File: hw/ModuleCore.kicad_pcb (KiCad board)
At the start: 2 copper layers, 38.1 x 99.1 mm, 24 parts, among them J6 power_bus, J8 Conn_02x09_Odd_Even, Q1 2SC1815, SW5 SW_Push, U1 TL074, U2 ProMicro, U3 74HC595

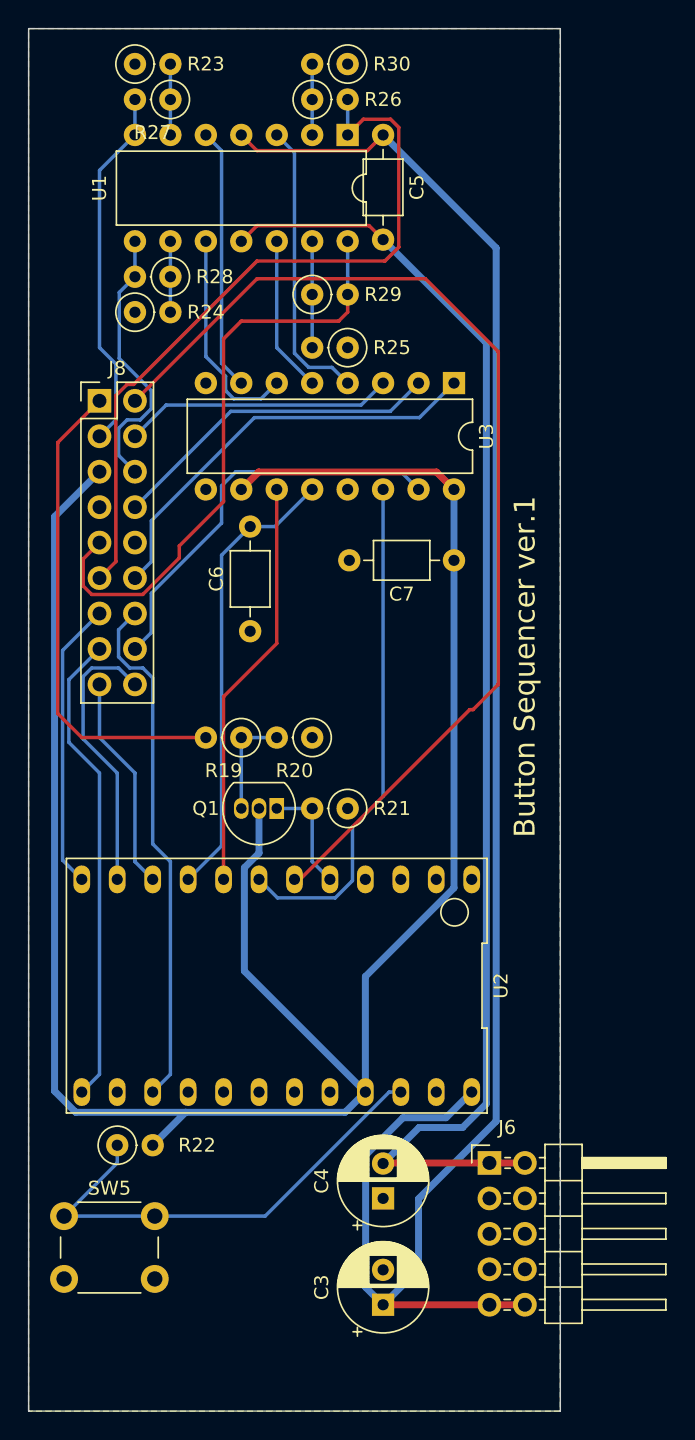
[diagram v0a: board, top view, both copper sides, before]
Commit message: minor mods
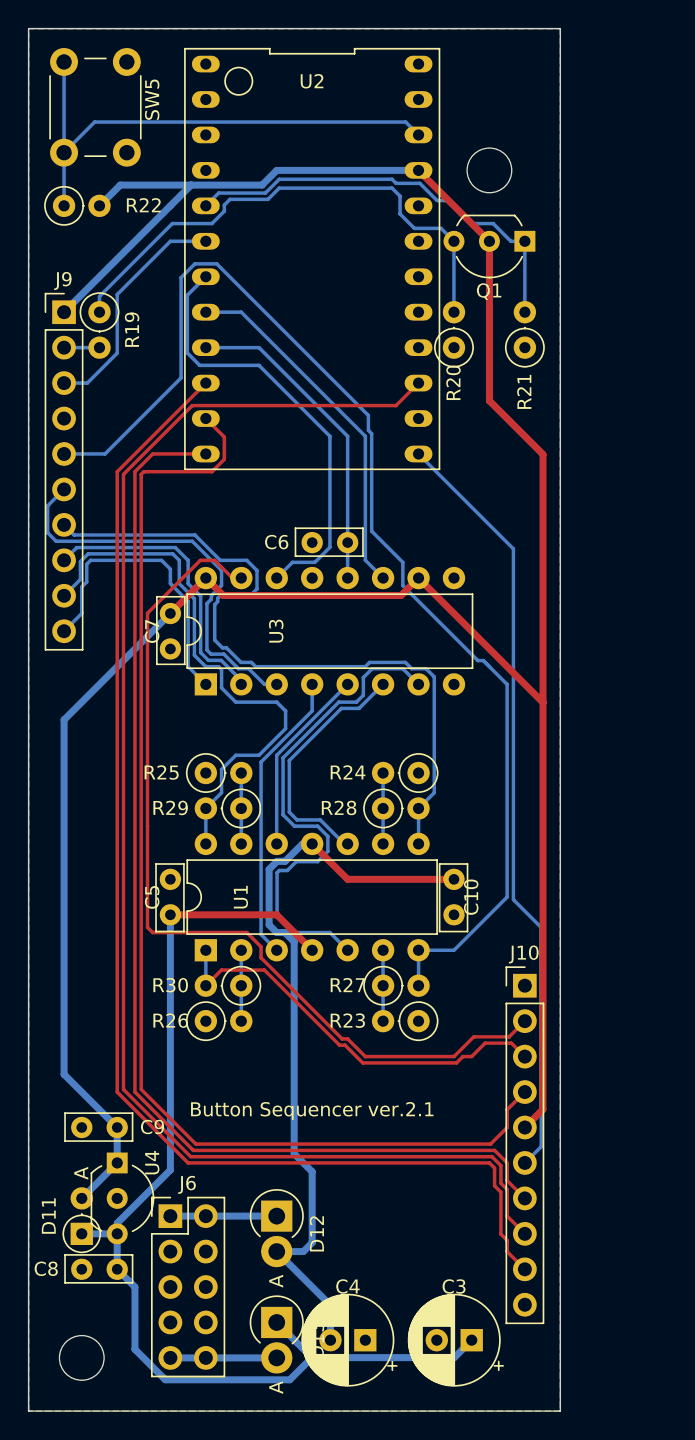
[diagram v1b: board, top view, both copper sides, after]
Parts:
- removed J8: Conn_02x09_Odd_Even, Connector_PinHeader_2.54mm:PinHeader_2x09_P2.54mm_Vertical
- added C10: 0.1u, Attenuverter:C_Axial_L4.8mm_D2.0mm_P2.54mm_Horizontal, F.Cu at (91.4, 104.1)
- added C8: 0.1u, Attenuverter:C_Axial_L4.8mm_D2.0mm_P2.54mm_Horizontal, F.Cu at (64.8, 129.5)
- added C9: 0.1u, Attenuverter:C_Axial_L4.8mm_D2.0mm_P2.54mm_Horizontal, F.Cu at (64.8, 119.4)
- added D11: 1N4148, Diode_THT:D_DO-35_SOD27_P2.54mm_Vertical_AnodeUp, F.Cu at (64.8, 127.0)
- added D12: D_Schottky, Diode_THT:D_DO-15_P2.54mm_Vertical_AnodeUp, F.Cu at (78.7, 125.7)
- added D13: D_Schottky, Diode_THT:D_DO-15_P2.54mm_Vertical_AnodeUp, F.Cu at (78.7, 133.3)
- added J10: bus_R, Connector_PinHeader_2.54mm:PinHeader_1x10_P2.54mm_Vertical, F.Cu at (96.5, 109.2)
- added J9: bus_L, Connector_PinHeader_2.54mm:PinHeader_1x10_P2.54mm_Vertical, F.Cu at (63.5, 61.0)
- added REF**: MountingHole_3.2mm_M3, MountingHole:MountingHole_3.2mm_M3, F.Cu at (94.0, 50.8)
- added REF**: MountingHole_3.2mm_M3, MountingHole:MountingHole_3.2mm_M3, F.Cu at (64.8, 135.9)
- added U4: L78L05_TO92, Package_TO_SOT_THT:TO-92_Inline_Wide, F.Cu at (67.3, 121.9)
- C5, C6, C7: footprint Capacitor_THT:C_Axial_L3.8mm_D2.6mm_P7.50mm_Horizontal -> Attenuverter:C_Axial_L4.8mm_D2.0mm_P2.54mm_Horizontal
- J6: footprint Connector_PinHeader_2.54mm:PinHeader_2x05_P2.54mm_Horizontal -> Connector_PinHeader_2.54mm:PinHeader_2x05_P2.54mm_Vertical
- Q1: footprint Package_TO_SOT_THT:TO-92_Inline -> Package_TO_SOT_THT:TO-92_Inline_Wide
- moved SW5 76.2 mm to (63.5, 49.5), turned to 90 degrees
- moved R23 71.5 mm to (88.9, 111.8), turned to 180 degrees
- moved R26 69.3 mm to (73.7, 111.8), turned to 0 degrees
- moved R22 67.4 mm to (63.5, 53.3)
- moved R27 65.3 mm to (86.4, 109.2), turned to 0 degrees
- moved R30 63.7 mm to (76.2, 109.2), turned to 180 degrees
- moved U1 59.3 mm to (73.7, 106.7), turned to 90 degrees
- moved C5 57.9 mm to (71.1, 104.1), turned to 90 degrees
- moved U2 52.1 mm to (81.3, 57.1), turned to 270 degrees
- moved Q1 44.4 mm to (96.5, 55.9)
- moved R28 41.0 mm to (86.4, 96.5), turned to 0 degrees
- moved R24 38.8 mm to (88.9, 94.0), turned to 180 degrees
- moved R29 37.2 mm to (76.2, 96.5), turned to 180 degrees
- moved R21 35.4 mm to (96.5, 63.5), turned to 90 degrees
- moved R19 32.1 mm to (66.0, 61.0), turned to 270 degrees
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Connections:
- C5 pad 2: -12V -> GND
- J6 pad 1: -12V -> Net-(D12-Pad1)
- J6 pad 10: +12V -> Net-(D13-Pad2)
- J6 pad 2: -12V -> Net-(D12-Pad1)
- J6 pad 9: +12V -> Net-(D13-Pad2)
- U2 pad 24: +12V -> Net-(U2-Pad24)
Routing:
- net /Sheet62451AD7/sw_enter: track 15.5 -> 90.9 mm
- net /Sheet62451AD7/sw_func_1: track 20.0 -> 85.5 mm
- net /Sheet62451AD7/sw_func_2: track 37.4 -> 102.8 mm
- net /Sheet62451AD7/re_1: track 20.7 -> 81.9 mm
- net /Sheet62451AD7/gate_1: track 26.2 -> 85.9 mm
- net /Sheet62451AD7/seq_start: track 76.1 -> 16.8 mm
- net +12V: track 132.5 -> 76.8 mm
- net -12V: track 95.4 -> 54.2 mm
- net /Sheet62451AD7/select_4: track 29.3 -> 63.7 mm
- net /Sheet62451AD7/clock_in: track 35.0 -> 2.54 mm
- net /Sheet62451AD7/gate_2: track 19.9 -> 52.2 mm
- net +5V: track 159.0 -> 189.8 mm
- net Net-(Q1-Pad3): track 7.62 -> 37.4 mm
- net /Sheet62451AD7/gate_4: track 53.7 -> 29.6 mm
- net /Sheet62451AD7/clock: track 8.15 -> 30.6 mm
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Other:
- board text added: "Button Sequencer ver.2.1"
- board text removed: "Button Sequencer ver.1"
